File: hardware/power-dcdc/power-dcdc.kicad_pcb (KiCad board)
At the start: 2 copper layers, 110 x 70 mm, 69 parts, among them J1 SOLAR_IN, J2 DCDC-MEASURES, J3 DCDC-PWM, J4 BATT2, J5 BATT1, Q1 SIR164ADP, Q2 SIR164ADP, Q3 SI7149ADP, Q4 SI7149ADP, Q5 SI7149ADP, Q6 SI7149ADP, U1 LP4951C, U2 NCP5901B, U3 PAC1953-1, U4 DGD0215, U5 DGD0215

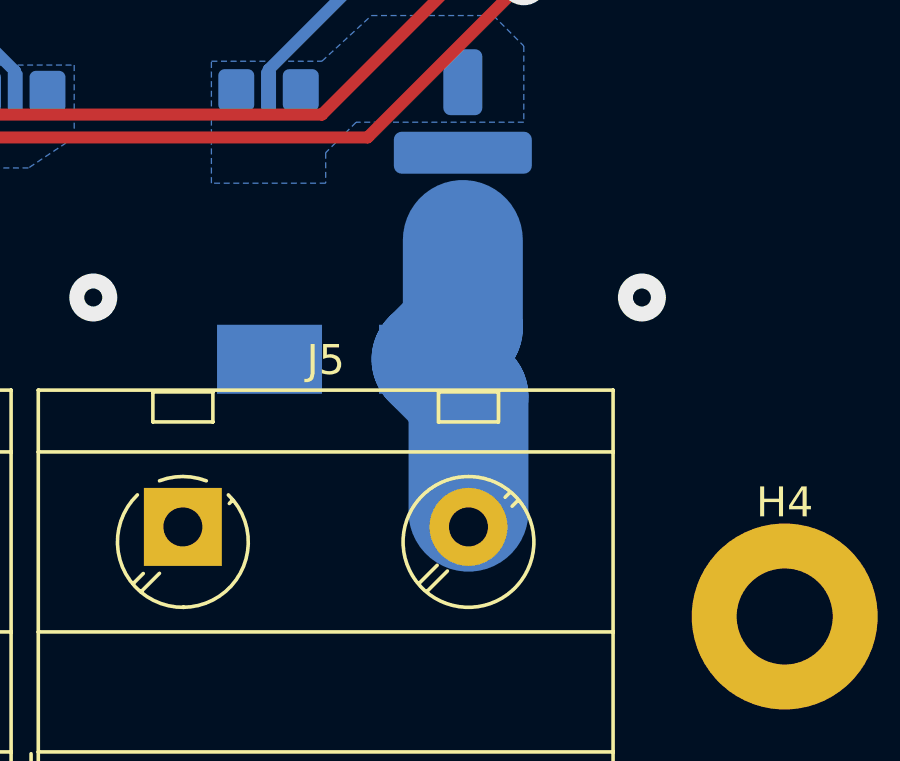
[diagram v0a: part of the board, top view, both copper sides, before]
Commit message: one more track cleanup
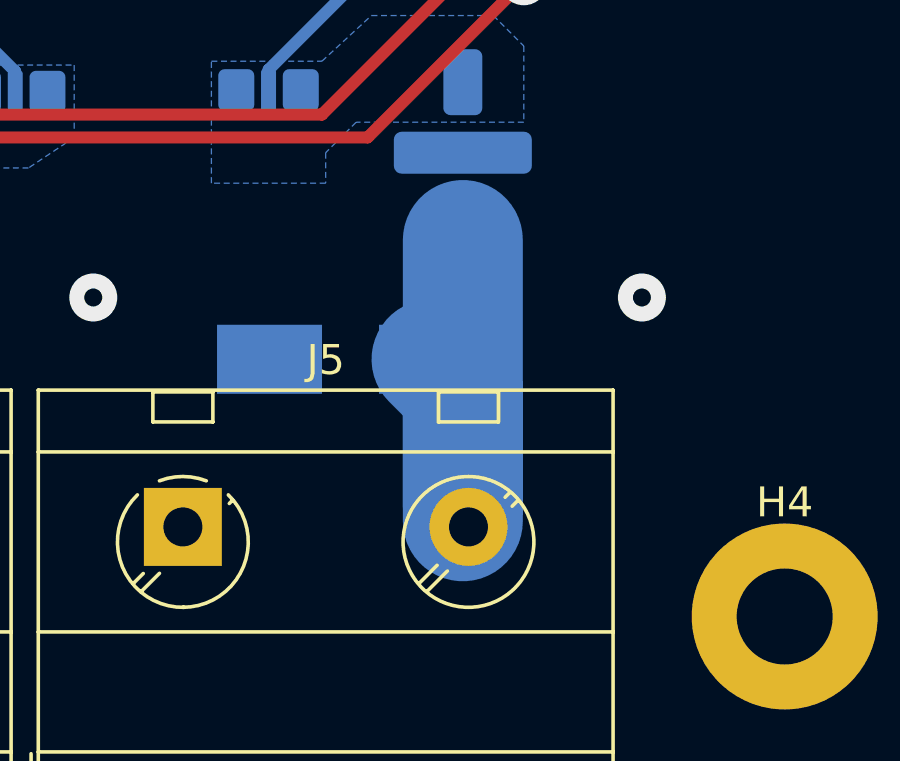
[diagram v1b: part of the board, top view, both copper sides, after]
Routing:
- net Net-(C16-Pad1): track 10.00 -> 14.7 mm
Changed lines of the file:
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@@
   (segment (start 121.981 119.6395) (end 124.058 119.6395) (width 0.6) (layer "B.Cu") (net 11))
   (segment (start 126.365 113.8055) (end 126.365 117.856) (width 0.6) (layer "B.Cu") (net 11))
-  (segment (start 144.46 141.506) (end 144.46 137.658) (width 4) (layer "B.Cu") (net 12))
-  (segment (start 143.228 136.426) (end 144.272 135.382) (width 4) (layer "B.Cu") (net 12))
-  (segment (start 144.272 135.382) (end 144.272 132.45) (width 4) (layer "B.Cu") (net 12))
-  (segment (start 144.46 137.658) (end 143.228 136.426) (width 4) (layer "B.Cu") (net 12))
+  (segment (start 144.272 137.47) (end 143.228 136.426) (width 4) (layer "B.Cu") (net 12))
+  (segment (start 144.272 141.826) (end 144.272 132.45) (width 4) (layer "B.Cu") (net 12))
+  (segment (start 144.272 141.318) (end 144.272 137.47) (width 4) (layer "B.Cu") (net 12))
   (segment (start 143.6635 109.474) (end 143.6635 111.551) (width 0.6) (layer "B.Cu") (net 13))
   (segment (start 143.3885 111.826) (end 145.6635 111.826) (width 0.6) (layer "B.Cu") (net 13))
